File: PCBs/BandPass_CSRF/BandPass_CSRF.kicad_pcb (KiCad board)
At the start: 2 copper layers, 41.9 x 20.3 mm, 10 parts, among them J1 Conn_Coaxial, J2 Conn_Coaxial

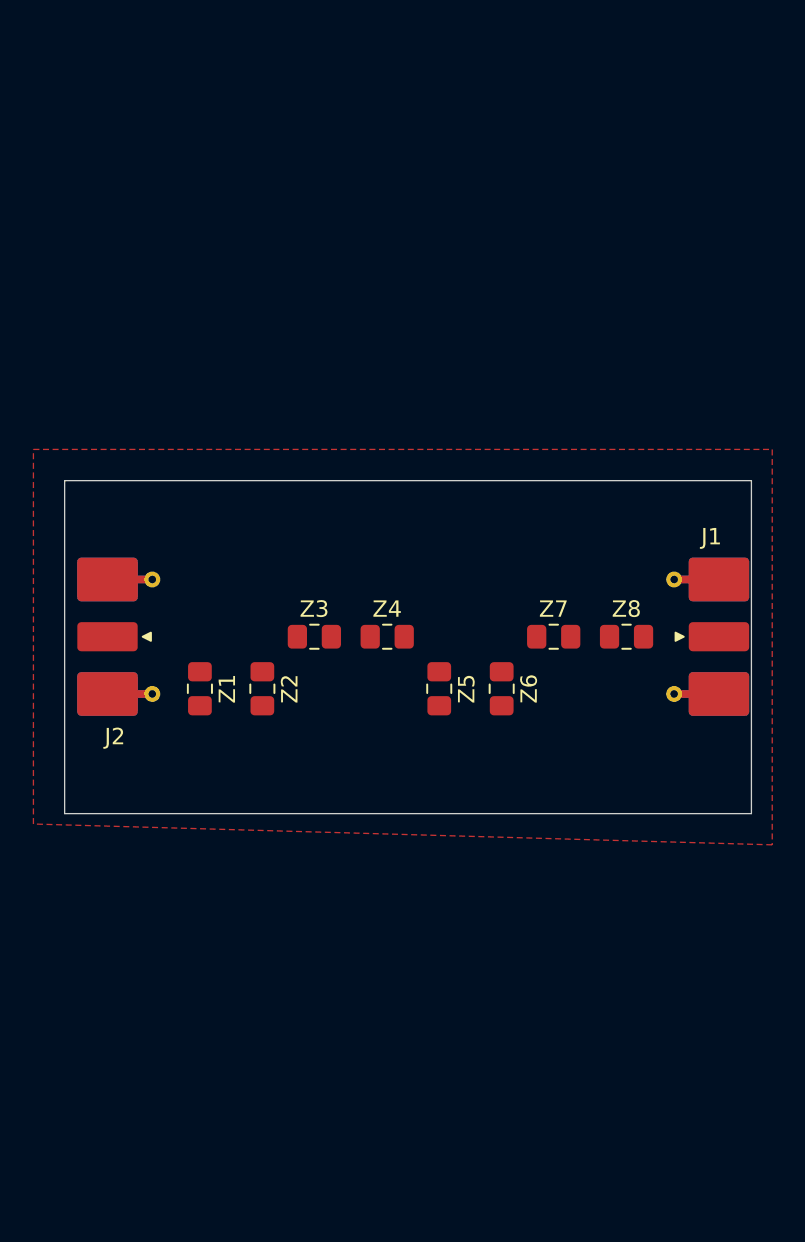
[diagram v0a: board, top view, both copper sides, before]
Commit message: one and done
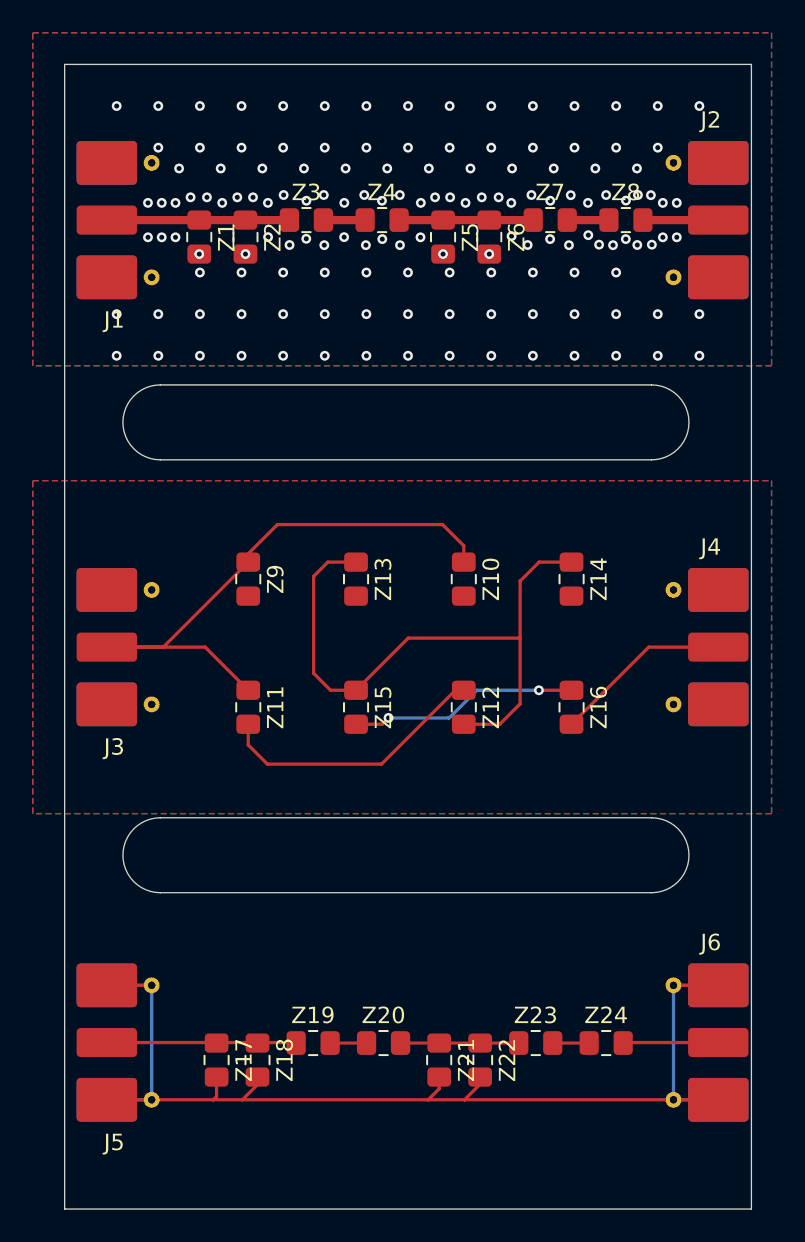
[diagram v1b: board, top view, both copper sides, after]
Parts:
- added J3: Conn_Coaxial, Connector_Coaxial:SMA_Molex_73251-2120_EdgeMount_Horizontal, F.Cu at (108.4, 86.4)
- added J4: Conn_Coaxial, Connector_Coaxial:SMA_Molex_73251-2120_EdgeMount_Horizontal, F.Cu at (146.2, 86.4)
- added J5: Conn_Coaxial, Connector_Coaxial:SMA_Molex_73251-2120_EdgeMount_Horizontal, F.Cu at (108.4, 110.5)
- added J6: Conn_Coaxial, Connector_Coaxial:SMA_Molex_73251-2120_EdgeMount_Horizontal, F.Cu at (146.2, 110.5)
- added Z10: L, Capacitor_SMD:C_0805_2012Metric_Pad1.18x1.45mm_HandSolder, F.Cu at (130.4, 82.2)
- added Z11: C, Capacitor_SMD:C_0805_2012Metric_Pad1.18x1.45mm_HandSolder, F.Cu at (117.2, 90.0)
- added Z12: L, Capacitor_SMD:C_0805_2012Metric_Pad1.18x1.45mm_HandSolder, F.Cu at (130.4, 90.0)
- added Z13: C, Capacitor_SMD:C_0805_2012Metric_Pad1.18x1.45mm_HandSolder, F.Cu at (123.8, 82.2)
- added Z14: L, Capacitor_SMD:C_0805_2012Metric_Pad1.18x1.45mm_HandSolder, F.Cu at (137.0, 82.2)
- added Z15: C, Capacitor_SMD:C_0805_2012Metric_Pad1.18x1.45mm_HandSolder, F.Cu at (123.8, 90.0)
- added Z16: L, Capacitor_SMD:C_0805_2012Metric_Pad1.18x1.45mm_HandSolder, F.Cu at (137.0, 90.0)
- added Z17: C, Capacitor_SMD:C_0805_2012Metric_Pad1.18x1.45mm_HandSolder, F.Cu at (115.3, 111.6)
- added Z18: L, Capacitor_SMD:C_0805_2012Metric_Pad1.18x1.45mm_HandSolder, F.Cu at (117.8, 111.6)
- added Z19: C, Capacitor_SMD:C_0805_2012Metric_Pad1.18x1.45mm_HandSolder, F.Cu at (121.2, 110.5)
- added Z20: L, Capacitor_SMD:C_0805_2012Metric_Pad1.18x1.45mm_HandSolder, F.Cu at (125.5, 110.5)
- added Z21: C, Capacitor_SMD:C_0805_2012Metric_Pad1.18x1.45mm_HandSolder, F.Cu at (128.9, 111.6)
- added Z22: L, Capacitor_SMD:C_0805_2012Metric_Pad1.18x1.45mm_HandSolder, F.Cu at (131.4, 111.6)
- added Z23: C, Capacitor_SMD:C_0805_2012Metric_Pad1.18x1.45mm_HandSolder, F.Cu at (134.8, 110.5)
- added Z24: L, Capacitor_SMD:C_0805_2012Metric_Pad1.18x1.45mm_HandSolder, F.Cu at (139.1, 110.5)
- added Z9: C, Capacitor_SMD:C_0805_2012Metric_Pad1.18x1.45mm_HandSolder, F.Cu at (117.2, 82.2)
- moved Z2 27.6 mm to (117.1, 61.3)
- moved Z6 27.6 mm to (132.0, 61.3)
- moved Z5 27.6 mm to (129.1, 61.3)
- moved Z1 27.6 mm to (114.3, 61.3)
- moved Z3 25.4 mm to (120.8, 60.3)
- moved Z4 25.4 mm to (125.4, 60.3)
- moved Z7 25.4 mm to (135.7, 60.3)
- moved J1 25.4 mm to (108.4, 60.3)
- moved J2 25.4 mm to (146.2, 60.3)
- moved Z8 25.4 mm to (140.3, 60.3)
- renumbered J2 to J1, J1 to J2
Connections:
- net /GND renamed /GND1
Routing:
- net /GND3: track 0.00 -> 74.4 mm
- net Net-(Z12-Pad2): track 0.00 -> 38.3 mm
- net Net-(J3-In): track 0.00 -> 36.4 mm
- net Net-(Z11-Pad2): track 0.00 -> 16.8 mm
- net Net-(Z15-Pad2): track 0.00 -> 14.0 mm, vias 0 -> 2
- net Net-(J5-In): track 0.00 -> 11.6 mm
- net Net-(J1-In): track 0.00 -> 11.1 mm
- net Net-(J4-In): track 0.00 -> 10.9 mm
- net Net-(Z4-Pad2): track 0.00 -> 8.18 mm
- net Net-(Z20-Pad2): track 0.00 -> 7.21 mm
- net Net-(J6-In): track 0.00 -> 5.82 mm
- net Net-(J2-In): track 0.00 -> 4.60 mm
- net Net-(Z7-Pad2): track 0.00 -> 2.54 mm
- net Net-(Z3-Pad2): track 0.00 -> 2.54 mm
- net Net-(Z19-Pad2): track 0.00 -> 2.22 mm
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- added copper zone on B.Cu, net /GND1
- added copper zone on B.Cu, net /GND2
- added copper zone on F.Cu, net /GND2
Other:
- board size 41.9 x 20.3 mm -> 41.9 x 69.9 mm
